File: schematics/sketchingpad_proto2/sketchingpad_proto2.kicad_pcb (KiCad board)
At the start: 4 copper layers, 158.5 x 66 mm, 83 parts, among them CN1 HC-1.0-4PWT, CN2 S2B-PH-SM4-TB, J1 AudioJack4, Q1 AO3415A, SW1 TC-S3601-3.5-260G-F0.6, SW2 MINI MSK12CO2, U1 TS20, U2 Seeeduino Xiao nRF52840

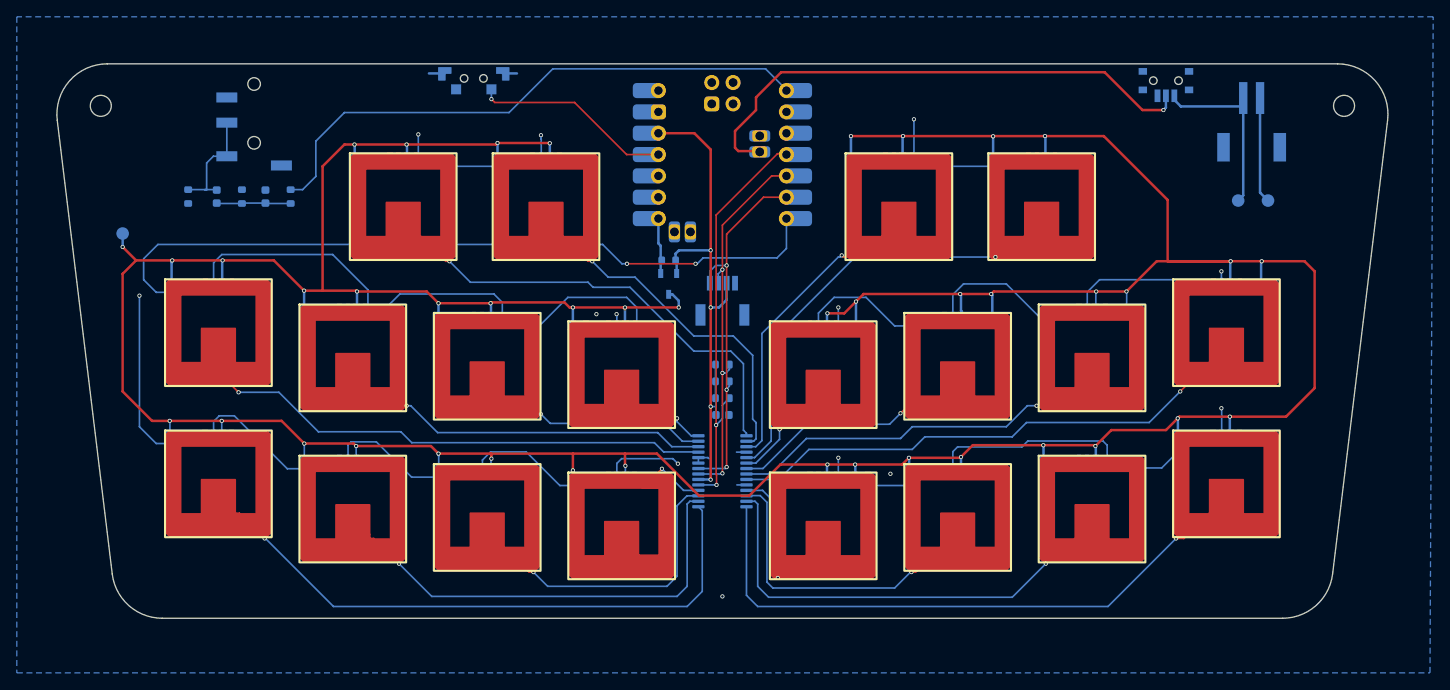
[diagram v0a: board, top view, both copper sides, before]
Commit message: front silk maybe
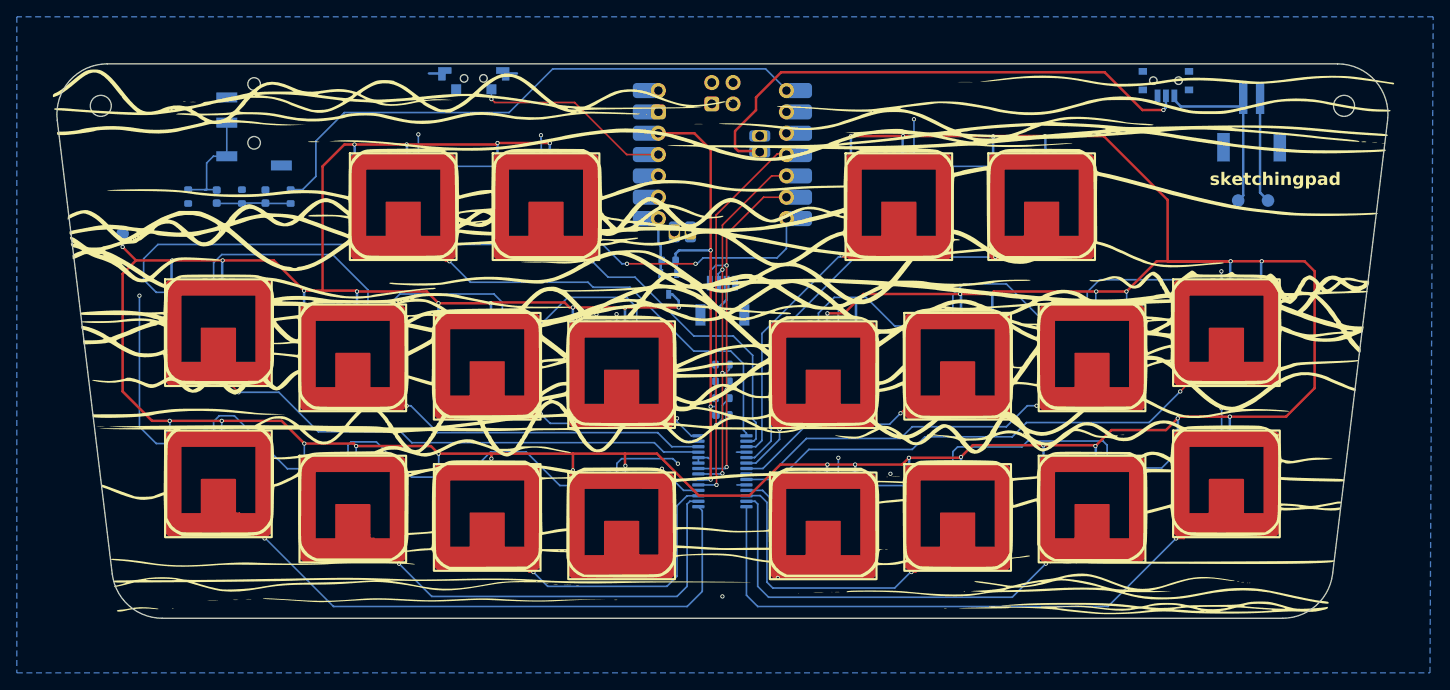
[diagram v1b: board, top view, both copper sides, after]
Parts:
- added G***: LOGO, LOGO, F.Cu at (136.0, 93.0)
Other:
- board text added: "sketchingpad"
